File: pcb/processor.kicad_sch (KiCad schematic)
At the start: 14 parts, among them U3 RP2040

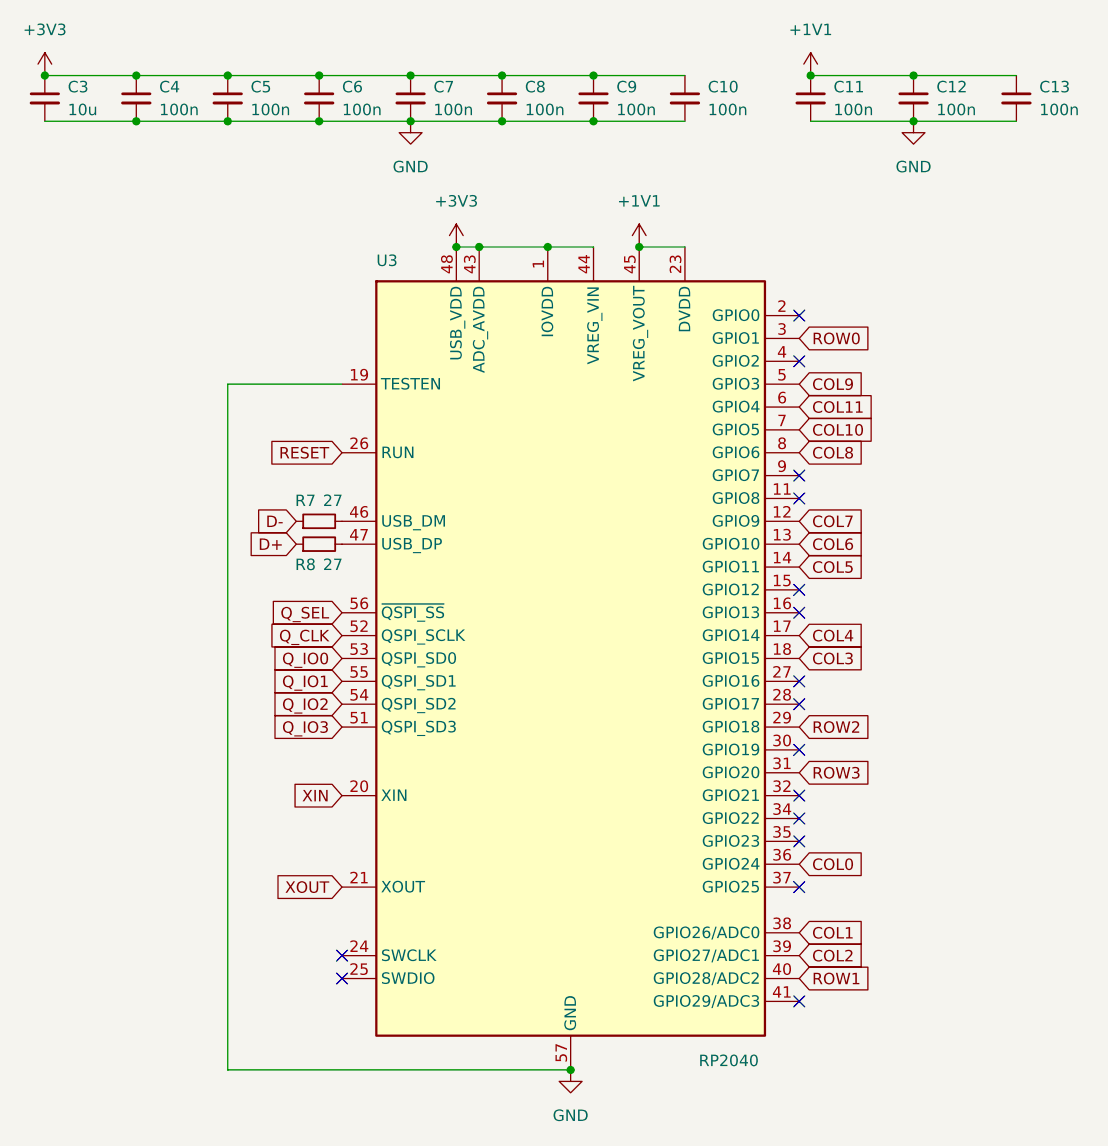
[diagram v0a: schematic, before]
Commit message: 2 layer final
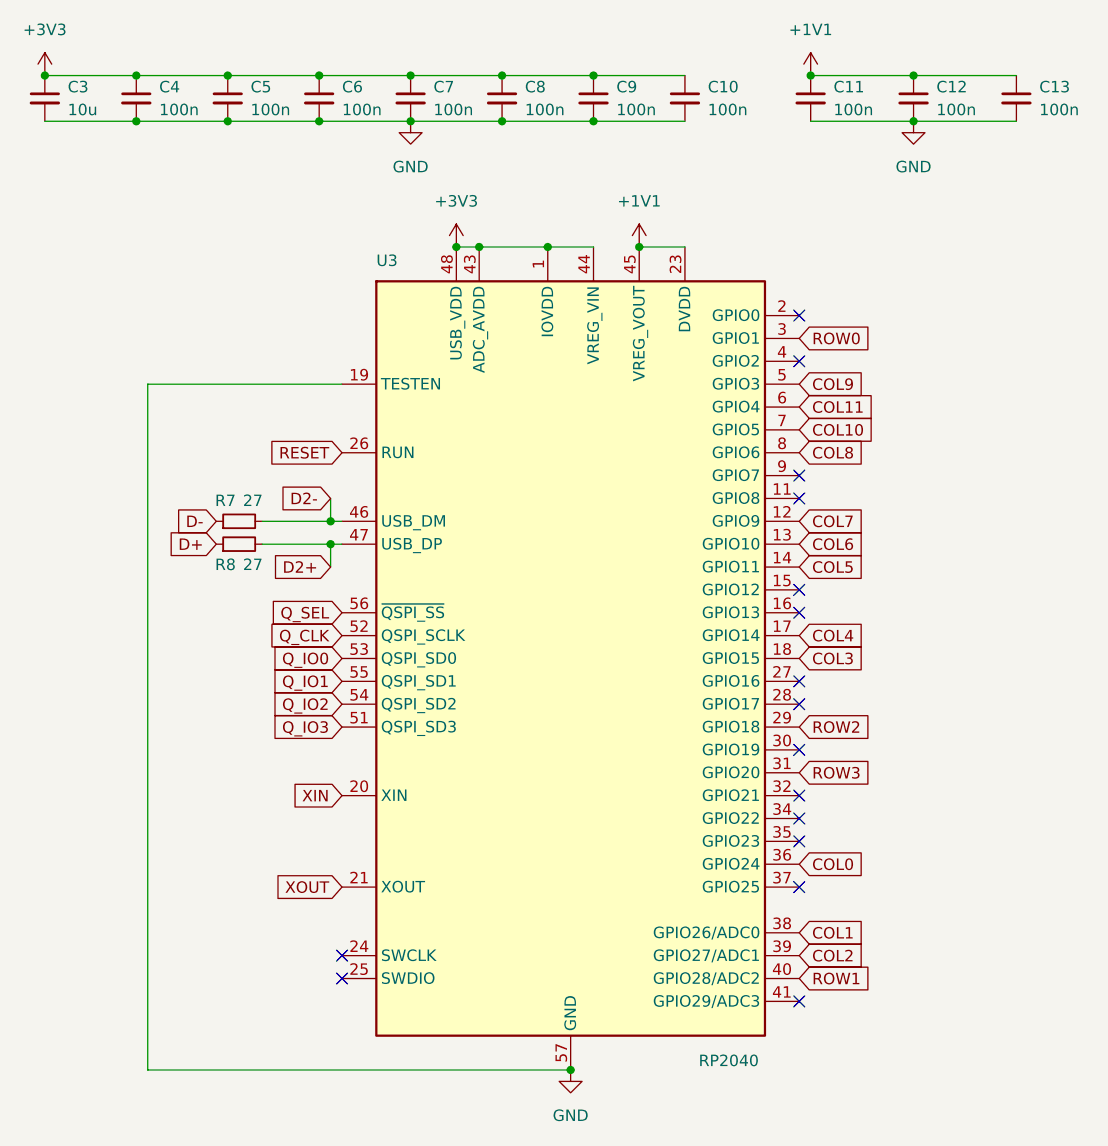
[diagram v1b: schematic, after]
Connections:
- net D2-: now reaches R7.2, U3.46 (USB_DM)
- net D2+: now reaches R8.2, U3.47 (USB_DP)
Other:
- moved on the sheet: R7, R8
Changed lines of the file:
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@@
+	)
+	(junction
+		(at 120.65 93.98)
+		(diameter 0)
+		(color 0 0 0 0)
 	)
 	(junction
@@
 		(color 0 0 0 0)
 	)
+	(junction
+		(at 120.65 96.52)
+		(diameter 0)
+		(color 0 0 0 0)
+	)
 	(no_connect
 		(at 121.92 144.78)
@@
 	(wire
 		(pts
+			(xy 113.03 96.52) (xy 120.65 96.52)
+		)
+		(stroke
+			(width 0)
+			(type default)
+		)
+	)
+	(wire
+		(pts
+			(xy 113.03 93.98) (xy 120.65 93.98)
+		)
+		(stroke
+			(width 0)
+			(type default)
+		)
+	)
+	(wire
+		(pts
 			(xy 129.54 44.45) (xy 139.7 44.45)
 		)
@@
 	(wire
 		(pts
-			(xy 121.92 78.74) (xy 109.22 78.74)
+			(xy 121.92 78.74) (xy 100.33 78.74)
+		)
+		(stroke
+			(width 0)
+			(type default)
+		)
+	)
+	(wire
+		(pts
+			(xy 120.65 99.06) (xy 120.65 96.52)
 		)
 		(stroke
@@
 	(wire
 		(pts
-			(xy 109.22 154.94) (xy 147.32 154.94)
+			(xy 100.33 154.94) (xy 147.32 154.94)
 		)
 		(stroke
@@
 	(wire
 		(pts
-			(xy 109.22 78.74) (xy 109.22 154.94)
+			(xy 100.33 78.74) (xy 100.33 154.94)
 		)
 		(stroke
@@
 	(wire
 		(pts
+			(xy 120.65 96.52) (xy 121.92 96.52)
+		)
+		(stroke
+			(width 0)
+			(type default)
+		)
+	)
+	(wire
+		(pts
+			(xy 120.65 93.98) (xy 121.92 93.98)
+		)
+		(stroke
+			(width 0)
+			(type default)
+		)
+	)
+	(wire
+		(pts
 			(xy 173.99 49.53) (xy 185.42 49.53)
 		)
@@
 		)
 	)
+	(wire
+		(pts
+			(xy 120.65 91.44) (xy 120.65 93.98)
+		)
+		(stroke
+			(width 0)
+			(type default)
+		)
+	)
 	(global_label "COL6"
 		(shape input)
@@
 	(global_label "D+"
 		(shape input)
-		(at 116.84 96.52 180)
+		(at 107.95 96.52 180)
 		(fields_autoplaced yes)
 		(effects
@@
 		)
 		(property "Intersheetrefs" "${INTERSHEET_REFS}"
-			(at 111.0124 96.52 0)
+			(at 102.1224 96.52 0)
 			(effects
 				(font
@@
 		)
 	)
+	(global_label "D2-"
+		(shape input)
+		(at 120.65 91.44 180)
+		(fields_autoplaced yes)
+		(effects
+			(font
+				(size 1.27 1.27)
+			)
+			(justify right)
+		)
+		(property "Intersheetrefs" "${INTERSHEET_REFS}"
+			(at 113.6129 91.44 0)
+			(effects
+				(font
+					(size 1.27 1.27)
+				)
+				(justify right)
+				(hide yes)
+			)
+		)
+	)
 	(global_label "RESET"
 		(shape input)
@@
 	(global_label "D-"
 		(shape input)
-		(at 116.84 93.98 180)
+		(at 107.95 93.98 180)
 		(fields_autoplaced yes)
 		(effects
@@
 		)
 		(property "Intersheetrefs" "${INTERSHEET_REFS}"
-			(at 111.0124 93.98 0)
+			(at 102.1224 93.98 0)
 			(effects
 				(font
@@
 				)
 				(justify left)
+				(hide yes)
+			)
+		)
+	)
+	(global_label "D2+"
+		(shape input)
+		(at 120.65 99.06 180)
+		(fields_autoplaced yes)
+		(effects
+			(font
+				(size 1.27 1.27)
+			)
+			(justify right)
+		)
+		(property "Intersheetrefs" "${INTERSHEET_REFS}"
+			(at 113.6129 99.06 0)
+			(effects
+				(font
+					(size 1.27 1.27)
+				)
+				(justify right)
 				(hide yes)
 			)
@@
 	(symbol
 		(lib_id "Device:R_Small")
-		(at 119.38 96.52 90)
+		(at 110.49 96.52 90)
 		(unit 1)
 		(exclude_from_sim no)
@@
 		(dnp no)
 		(property "Reference" "R8"
-			(at 117.856 98.806 90)
+			(at 108.966 98.806 90)
 			(effects
 				(font
@@
 		)
 		(property "Value" "27"
-			(at 120.904 98.806 90)
+			(at 112.014 98.806 90)
 			(effects
 				(font
@@
 		)
 		(property "Footprint" "Library:R_0402_1005Metric"
-			(at 119.38 96.52 0)
+			(at 110.49 96.52 0)
 			(effects
 				(font
@@
 		)
 		(property "Datasheet" "kicad-embed://C25100.pdf"
-			(at 119.38 96.52 0)
+			(at 110.49 96.52 0)
 			(effects
 				(font
@@
 		)
 		(property "Description" "Resistor, small symbol"
-			(at 119.38 96.52 0)
+			(at 110.49 96.52 0)
 			(effects
 				(font
@@
 		)
 		(property "LCSC" "C25100"
-			(at 119.38 96.52 90)
+			(at 110.49 96.52 90)
 			(effects
 				(font
@@
 		)
 		(property "KLC_S3.3" ""
-			(at 119.38 96.52 90)
+			(at 110.49 96.52 90)
 			(effects
 				(font
@@
 		)
 		(property "KLC_S4.1" ""
-			(at 119.38 96.52 90)
+			(at 110.49 96.52 90)
 			(effects
 				(font
@@
 		)
 		(property "KLC_S4.2_DVDD" ""
-			(at 119.38 96.52 90)
+			(at 110.49 96.52 90)
 			(effects
 				(font
@@
 		)
 		(property "KLC_S4.2_VREG_VOUT" ""
-			(at 119.38 96.52 90)
+			(at 110.49 96.52 90)
 			(effects
 				(font
@@
 	(symbol
 		(lib_id "Device:R_Small")
-		(at 119.38 93.98 90)
+		(at 110.49 93.98 90)
 		(unit 1)
 		(exclude_from_sim no)
@@
 		(dnp no)
 		(property "Reference" "R7"
-			(at 117.856 91.694 90)
+			(at 108.966 91.694 90)
 			(effects
 				(font
@@
 		)
 		(property "Value" "27"
-			(at 120.904 91.694 90)
+			(at 112.014 91.694 90)
 			(effects
 				(font
@@
 		)
 		(property "Footprint" "Library:R_0402_1005Metric"
-			(at 119.38 93.98 0)
+			(at 110.49 93.98 0)
 			(effects
 				(font
@@
 		)
 		(property "Datasheet" "kicad-embed://C25100.pdf"
-			(at 119.38 93.98 0)
+			(at 110.49 93.98 0)
 			(effects
 				(font
@@
 		)
 		(property "Description" "Resistor, small symbol"
-			(at 119.38 93.98 0)
+			(at 110.49 93.98 0)
 			(effects
 				(font
@@
 		)
 		(property "LCSC" "C25100"
-			(at 119.38 93.98 90)
+			(at 110.49 93.98 90)
 			(effects
 				(font
@@
 		)
 		(property "KLC_S3.3" ""
-			(at 119.38 93.98 90)
+			(at 110.49 93.98 90)
 			(effects
 				(font
@@
 		)
 		(property "KLC_S4.1" ""
-			(at 119.38 93.98 90)
+			(at 110.49 93.98 90)
 			(effects
 				(font
@@
 		)
 		(property "KLC_S4.2_DVDD" ""
-			(at 119.38 93.98 90)
+			(at 110.49 93.98 90)
 			(effects
 				(font
@@
 		)
 		(property "KLC_S4.2_VREG_VOUT" ""
-			(at 119.38 93.98 90)
-			(effects
-				(font
+			(at 110.49 93.98 90)
+			(effects
+				(font
